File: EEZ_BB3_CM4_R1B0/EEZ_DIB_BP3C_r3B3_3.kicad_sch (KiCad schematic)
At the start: 22 parts, among them X4 DS1022-2*20RF11, X5 DS1023-2*14S21, X6 DS1023-2*14S21, X7 DS1023-2*14S21

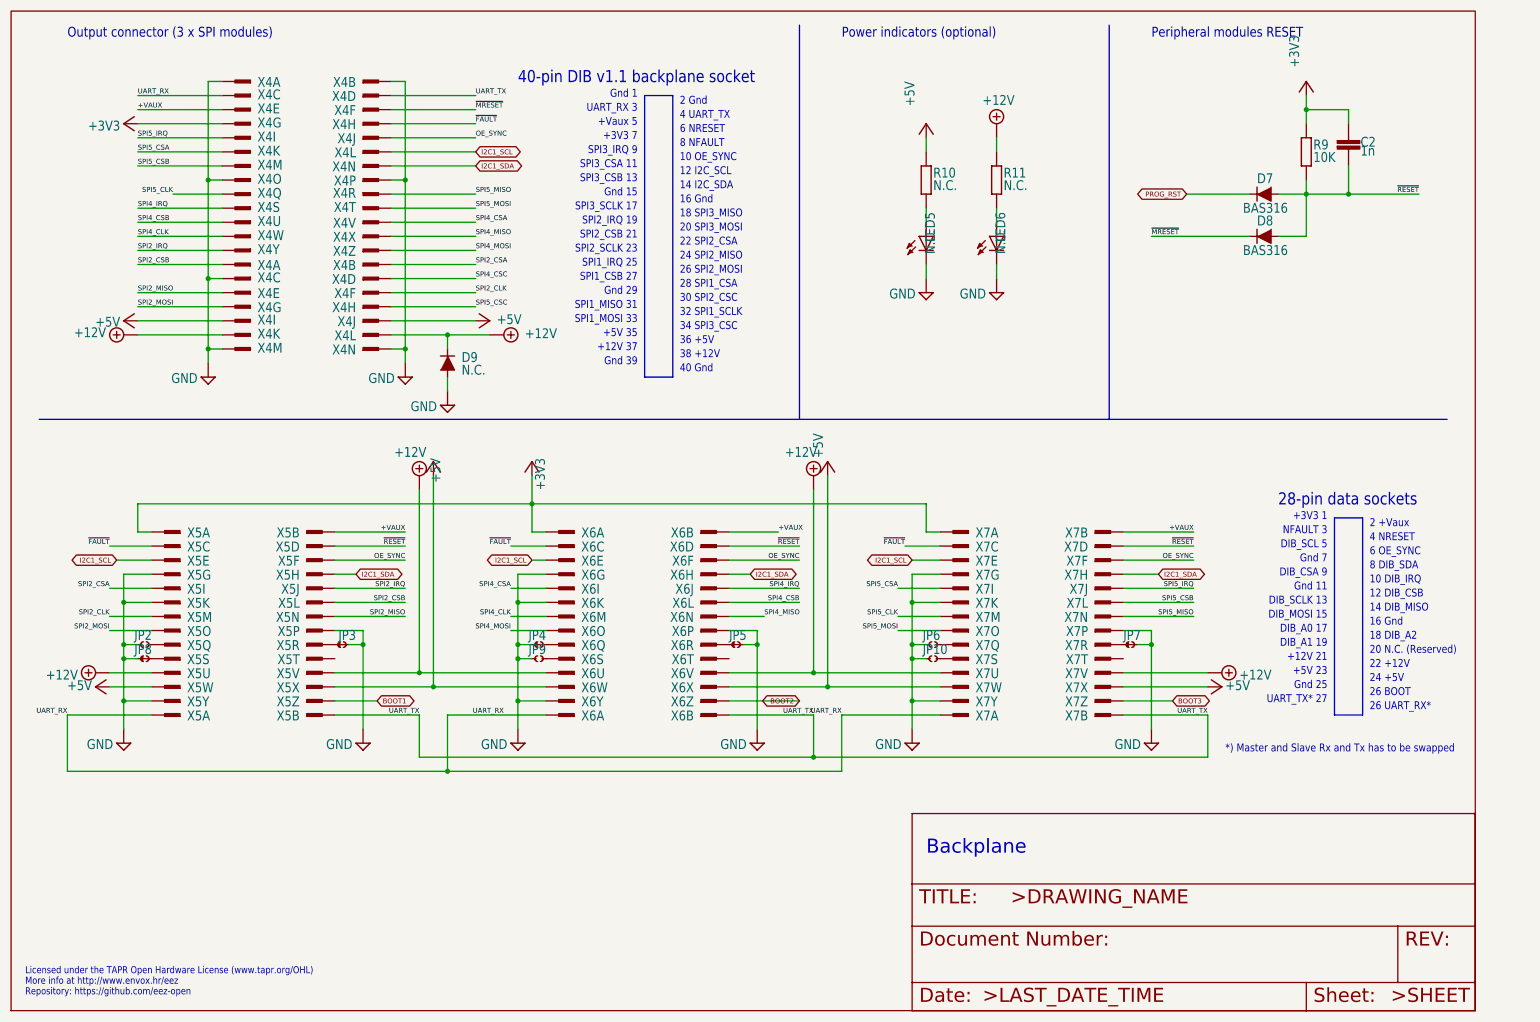
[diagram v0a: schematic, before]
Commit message: Importing BP3
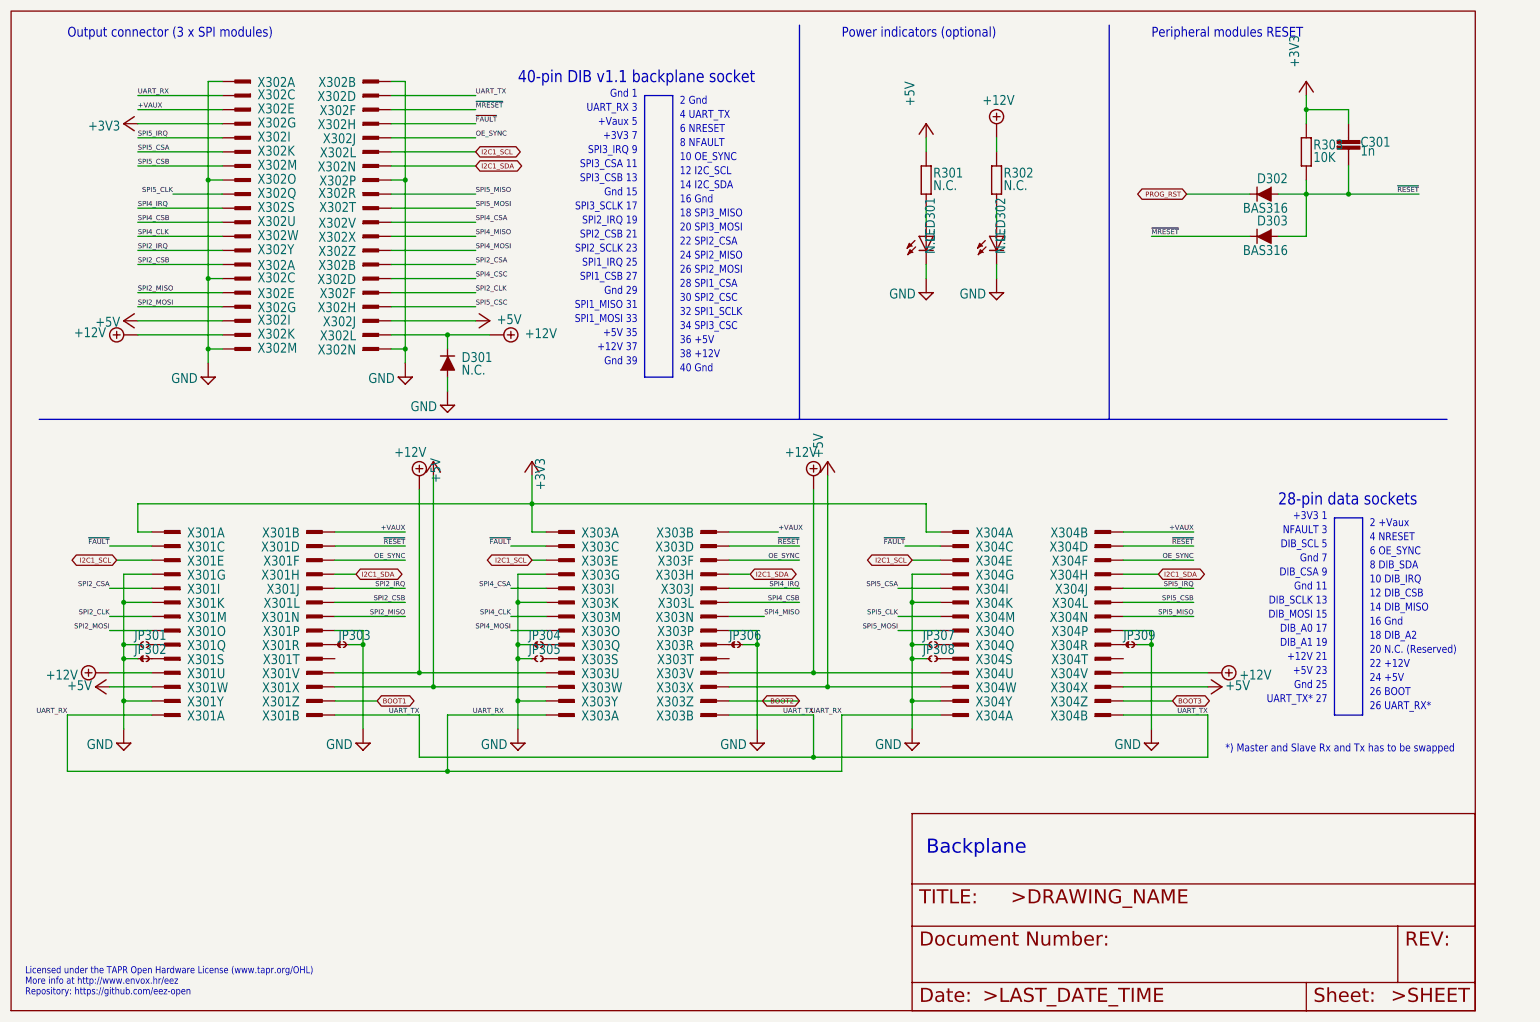
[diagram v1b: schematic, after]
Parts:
- renumbered C2 to C301, D9 to D301, D7 to D302, D8 to D303, JP2 to JP301, JP8 to JP302, JP3 to JP303, JP4 to JP304, JP9 to JP305, JP5 to JP306, JP6 to JP307, JP10 to JP308, JP7 to JP309, LED5 to LED301, LED6 to LED302, R10 to R301, R11 to R302, R9 to R303, X5 to X301, X4 to X302, X6 to X303, X7 to X304
